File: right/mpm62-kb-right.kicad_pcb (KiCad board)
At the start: 2 copper layers, 161.9 x 95.2 mm, 71 parts, among them J1 Conn_01x04_Male, J2 Conn_01x02_Male, U1 MCP23018-E_SP

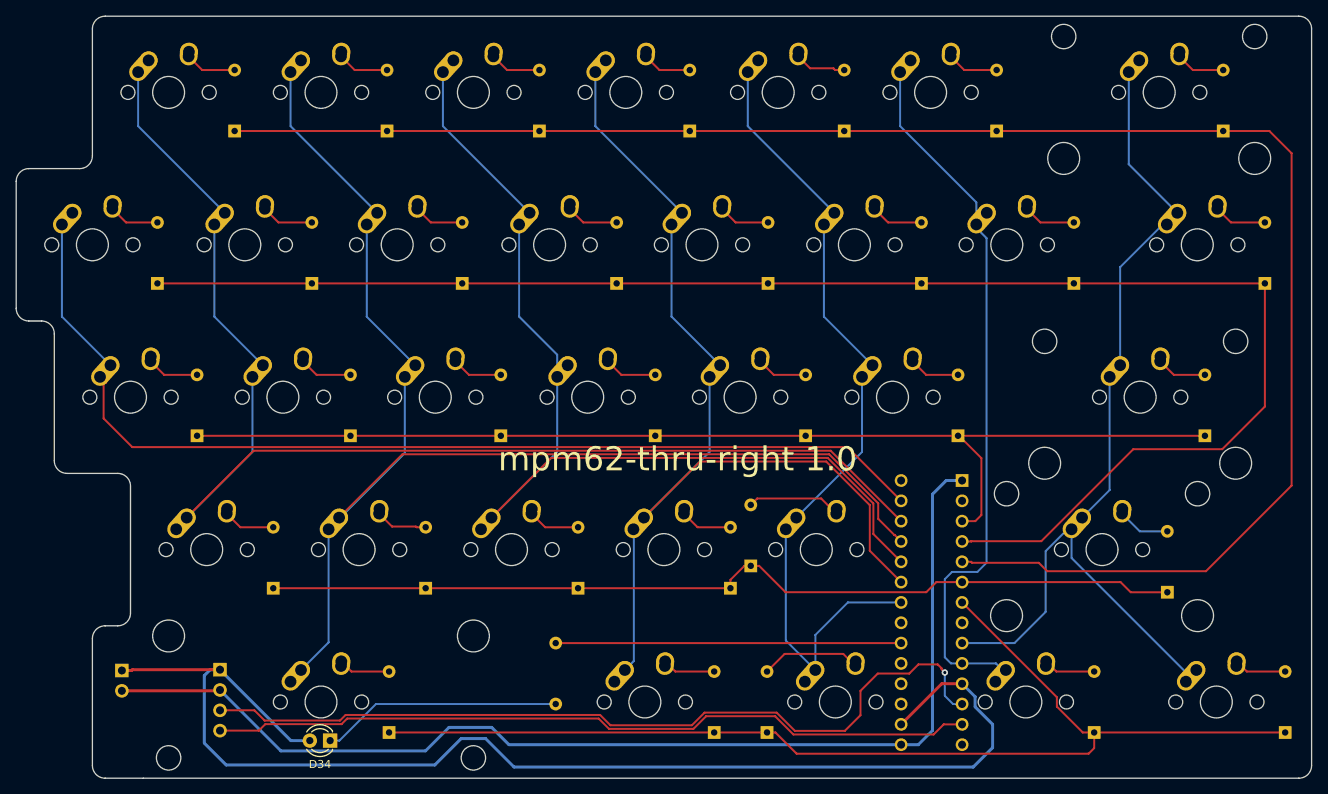
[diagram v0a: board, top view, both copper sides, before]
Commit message: Final for b1t (board 1 thruhole) board
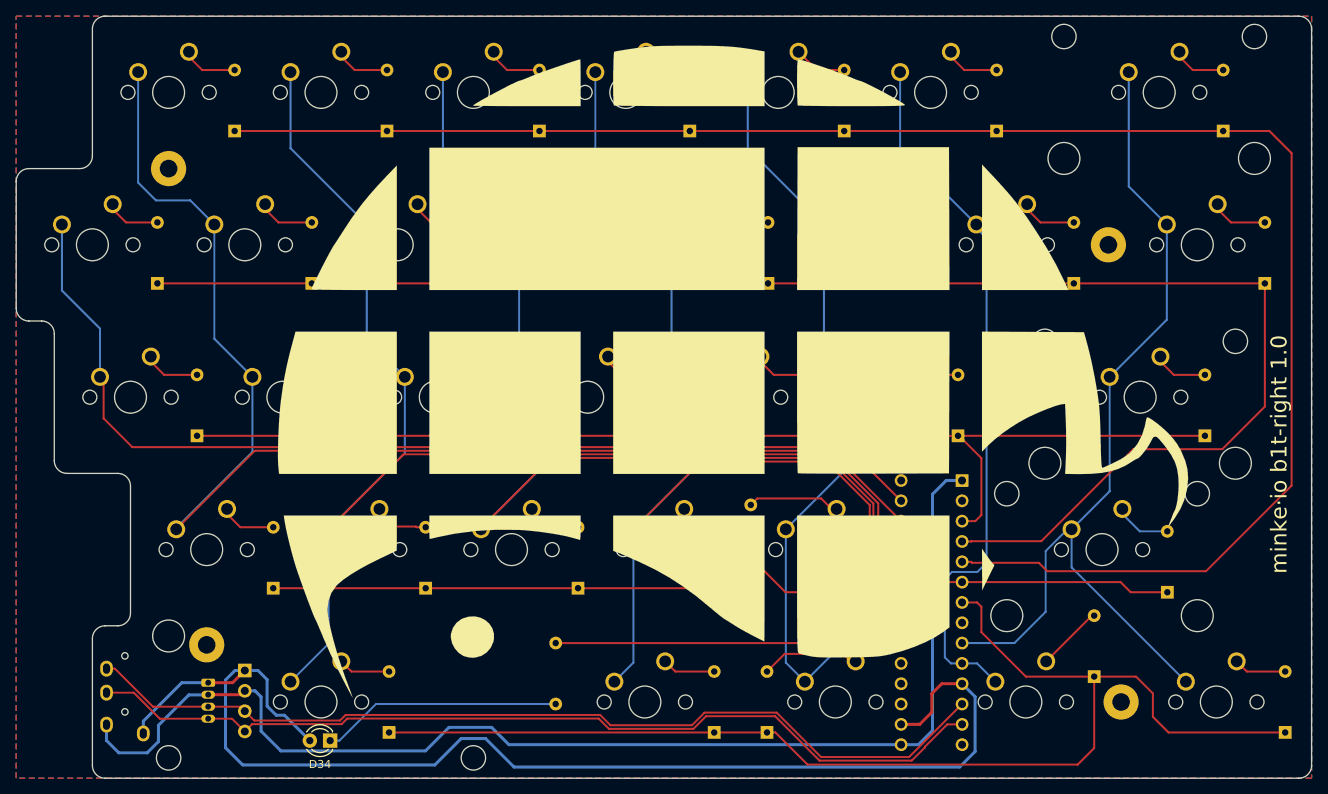
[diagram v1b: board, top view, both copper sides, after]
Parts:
- added G***: LOGO, MpmMisc:small_logo, B.Cu at (98.4, 124.6)
- added G***: LOGO, MpmMisc:biglogo3, F.Cu at (136.5, 92.6)
- added H1: MountingHole, MountingHole:MountingHole_2.2mm_M2_Pad, B.Cu at (66.7, 66.7)
- added H2: MountingHole, MountingHole:MountingHole_2.2mm_M2_Pad, B.Cu at (71.4, 126.2)
- added H3: MountingHole, MountingHole:MountingHole_2.2mm_M2_Pad, B.Cu at (184.2, 76.2)
- added H4: MountingHole, MountingHole:MountingHole_2.2mm_M2_Pad, B.Cu at (185.7, 133.3)
- added U2: TRRS, Keebio-Parts:TRRS-PJ-320A, B.Cu at (61.2, 126.0)
- J1: value Conn_01x04_Male -> Raw Header
- J2: value Conn_01x02_Male -> JST ZH Header; footprint Connector_PinHeader_2.54mm:PinHeader_1x02_P2.54mm_Vertical -> MpmMisc:JST_ZH_B4B-ZR_1x04_P1.50mm_Vertical
- MX1, MX10, MX12, MX13, MX14, MX15, MX16, MX17, MX18, MX19, MX2, MX21, MX22, MX23, MX24, MX26, MX27, MX3, MX4, MX5, MX6, MX7, MX8, MX9: footprint MX_Alps_Hybrid:MX-1U-NoLED -> MX_Only:MXOnly-1U-NoLED
- MX11: footprint MX_Alps_Hybrid:MX-3U-ReversedStabilizers-NoLED -> MX_Only:MXOnly-3U-ReversedStabilizers-NoLED
- MX20, MX25, MX28, MX33: footprint MX_Alps_Hybrid:MX-1.25U-NoLED -> MX_Only:MXOnly-1.25U-NoLED
- MX29: footprint MX_Alps_Hybrid:MX-2U-NoLED -> MX_Only:MXOnly-2U-NoLED
- MX30: footprint MX_Alps_Hybrid:MX-1.5U-NoLED -> MX_Only:MXOnly-1.5U-NoLED
- MX31: footprint MX_Alps_Hybrid:MX-2.25U-NoLED -> MX_Only:MXOnly-2.25U-NoLED
- MX32: footprint MX_Alps_Hybrid:MX-2.75U-NoLED -> MX_Only:MXOnly-2.75U-NoLED
- moved J2 10.9 mm to (71.6, 130.9), turned to 270 degrees
- moved D28 6.98 mm to (182.4, 130.2)
- moved J1 3.10 mm to (76.2, 129.4)
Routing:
- net Net-(J1-Pad4): track 96.0 -> 115.0 mm
- net Net-(J1-Pad3): track 104.8 -> 116.2 mm, vias 1 -> 0
- net GND: track 141.3 -> 152.7 mm
- net ROW4: track 139.3 -> 150.3 mm
- net COL11: track 125.9 -> 133.6 mm
- net COL8: track 161.6 -> 167.9 mm
- net COL9: track 163.4 -> 169.1 mm
- net COL14: track 108.4 -> 113.0 mm
- net COL12: track 99.1 -> 103.2 mm
- net Net-(D28-Pad2): track 6.53 -> 8.37 mm
- net COL10: track 130.0 -> 130.9 mm
- net COL7: track 130.5 -> 131.4 mm
- net COL13: track 90.3 -> 89.6 mm
- added copper zone on B.Cu, net GND
- added copper zone on F.Cu, net GND
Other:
- board text added: "minke·io b1t-right 1.0"
- board text removed: "mpm62-thru-right 1.0"
